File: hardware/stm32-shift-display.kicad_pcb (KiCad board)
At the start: 2 copper layers, 93.5 x 48.3 mm, 117 parts, among them J1 HDR_SWD, J2 USB_C_Receptacle_USB2.0_16P, SW1 SW_PUSH, SW2 SW_PUSH, SW3 SW_PUSH, SW4 SW_PUSH, SW5 218-2LPSTR, U1 AMS1117-3.3, U10 74HC595, U11 74HC595, U12 SM420561N, U13 SM420561N, U14 SM420561N, U2 STM32F103C8T6, U3 74HC595, U4 74HC595, U5 74HC595, U6 SM420561N, U7 SM420561N, U8 SM420561N, U9 74HC595, X1 OT32258MJBA4SL, X2 OK322532.768KJBA4SL

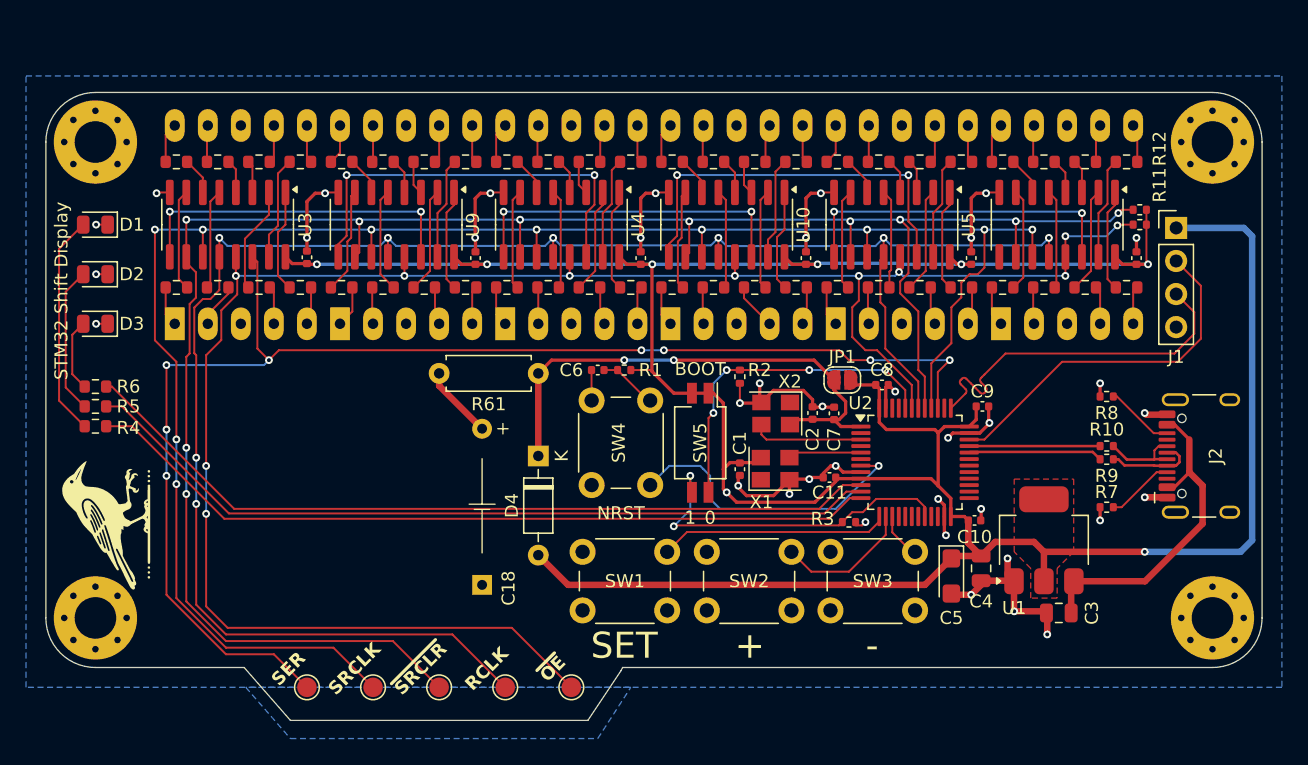
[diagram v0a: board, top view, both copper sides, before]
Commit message: Pre-autoroute on rev2
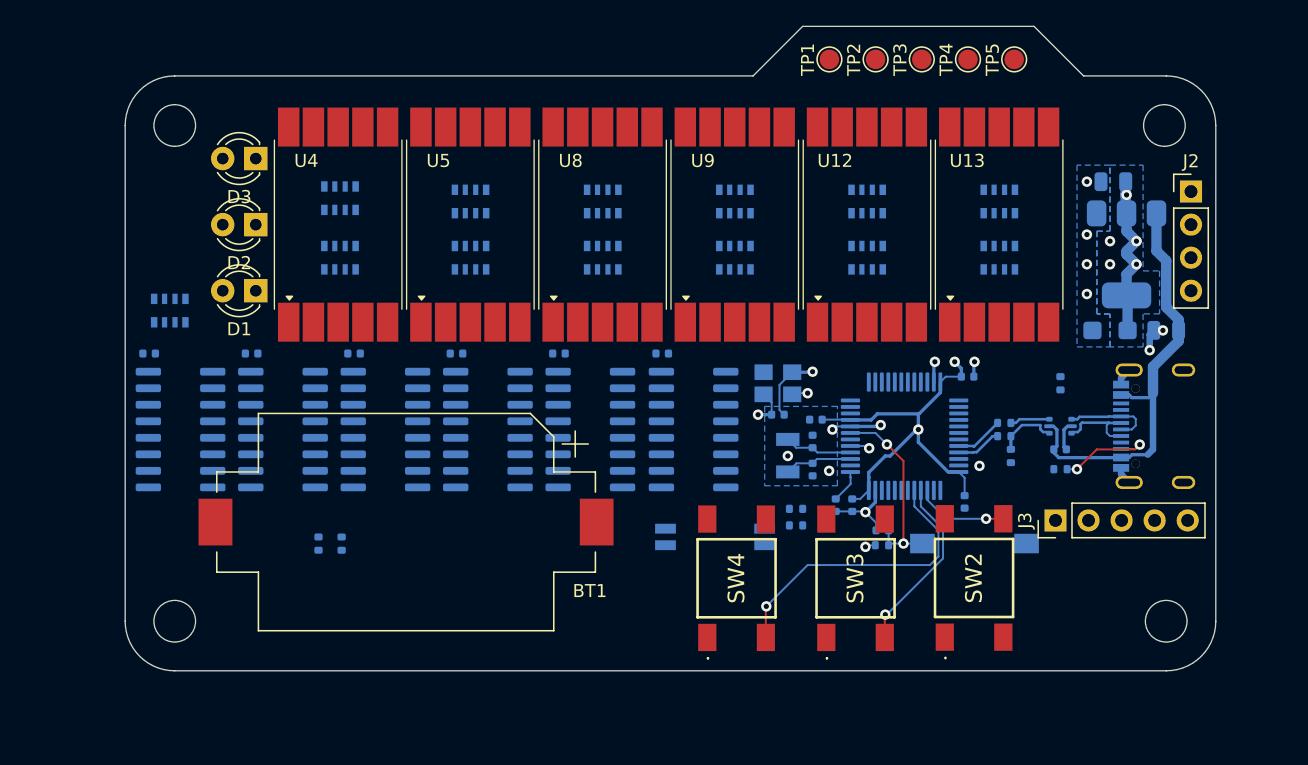
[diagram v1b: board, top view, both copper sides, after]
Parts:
- removed D4: BAT43, Diode_THT:D_DO-35_SOD27_P7.62mm_Horizontal
- removed G***: LOGO, CustomSymbols:GrackleLogo12mm
- removed JP1: SolderJumper_2_Open, Jumper:SolderJumper-2_P1.3mm_Open_RoundedPad1.0x1.5mm
- removed R10, R9: 10R, Resistor_SMD:R_0402_1005Metric
- removed R11: 10k, Resistor_SMD:R_0402_1005Metric
- removed R14, R15, R16, R17, R18, R19, R20, R21, R22, R23, R24, R25, R26, R27, R28, R29, R30, R31, R32, R33, R34, R35, R36, R37, R38, R39, R40, R41, R42, R43, R44, R45, R46, R47, R48, R49, R50, R51, R52, R53, R54, R55, R56, R57, R58, R59, R60: 470R, Resistor_SMD:R_0603_1608Metric
- removed R61: 22R, Resistor_THT:R_Axial_DIN0207_L6.3mm_D2.5mm_P7.62mm_Horizontal
- removed X2: OK322532.768KJBA4SL, Crystal:Crystal_SMD_3225-4Pin_3.2x2.5mm
- added BT1: 1060TR, Battery:BatteryHolder_Keystone_1060_1x2032, F.Cu at (144.8, 91.4)
- added C19: 100n, Capacitor_SMD:C_0402_1005Metric, B.Cu at (164.5, 78.5)
- added J3: HDR_UART, Connector_PinHeader_2.54mm:PinHeader_1x05_P2.54mm_Vertical, F.Cu at (194.7, 91.3)
- added RN1: 220R, Resistor_SMD:R_Array_Convex_4x0603, B.Cu at (139.7, 71.1)
- added RN10: 220R, Resistor_SMD:R_Array_Convex_4x0603, B.Cu at (190.4, 71.1)
- added RN11: 220R, Resistor_SMD:R_Array_Convex_4x0603, B.Cu at (180.2, 66.8)
- added RN12: 220R, Resistor_SMD:R_Array_Convex_4x0603, B.Cu at (190.4, 66.8)
- added RN13: 220R, Resistor_SMD:R_Array_Convex_4x0603, B.Cu at (126.6, 75.2)
- added RN2: 220R, Resistor_SMD:R_Array_Convex_4x0603, B.Cu at (149.7, 71.1)
- added RN3: 220R, Resistor_SMD:R_Array_Convex_4x0603, B.Cu at (139.7, 66.5)
- added RN4: 220R, Resistor_SMD:R_Array_Convex_4x0603, B.Cu at (149.7, 66.8)
- added RN5: 220R, Resistor_SMD:R_Array_Convex_4x0603, B.Cu at (159.9, 71.1)
- added RN6: 220R, Resistor_SMD:R_Array_Convex_4x0603, B.Cu at (170.1, 71.1)
- added RN7: 220R, Resistor_SMD:R_Array_Convex_4x0603, B.Cu at (159.9, 66.8)
- added RN8: 220R, Resistor_SMD:R_Array_Convex_4x0603, B.Cu at (170.1, 66.8)
- added RN9: 220R, Resistor_SMD:R_Array_Convex_4x0603, B.Cu at (180.2, 71.1)
- added U15: 74HC595, Package_SO:SOIC-16_3.9x9.9mm_P1.27mm, B.Cu at (166.9, 84.3)
- added Y1: Q13FC13500002, Crystal:Crystal_SMD_3215-2Pin_3.2x1.5mm, B.Cu at (174.1, 86.3)
- C1, C14, C15, C16, C17, C2, C6, C7, C8, R1, R12, SW5, U10, U11, U2, X1: moved to B.Cu
- C10, C9: value 100n -> 6p; moved to B.Cu
- C11, C12: footprint Capacitor_SMD:C_0402_1005Metric -> Capacitor_SMD:C_0805_2012Metric; moved to B.Cu
- C13: value 100n -> 10u; footprint Capacitor_SMD:C_0402_1005Metric -> Capacitor_Tantalum_SMD:CP_EIA-3216-18_Kemet-A; moved to B.Cu
- C18: value SCMR22C155PRBA0 -> 100n; footprint Mouser:SCMR22C155PRBA0 -> Capacitor_SMD:C_0402_1005Metric; moved to B.Cu
- C3, C4: footprint Capacitor_SMD:C_0805_2012Metric -> Capacitor_SMD:C_0402_1005Metric; moved to B.Cu
- C5: value 10u -> 100n; footprint Capacitor_Tantalum_SMD:CP_EIA-3216-18_Kemet-A -> Capacitor_SMD:C_0402_1005Metric; moved to B.Cu
- D1, D2, D3: value KT-0805Y -> LED_YLW; footprint LED_SMD:LED_0805_2012Metric -> LED_THT:LED_D3.0mm
- H1, H2, H3, H4: footprint MountingHole:MountingHole_3.2mm_M3_Pad_Via -> MountingHole:MountingHole_3.2mm_M3_ISO7380
- J1: value HDR_SWD -> GT-USB-7010ASV; footprint Connector_PinHeader_2.54mm:PinHeader_1x04_P2.54mm_Vertical -> easyeda2kicad:USB-C-SMD_G-SWITCH_GT-USB-7010ASV; moved to B.Cu
- J2: value USB_C_Receptacle_USB2.0_16P -> HDR_SWD; footprint Connector_USB:USB_C_Receptacle_HCTL_HC-TYPE-C-16P-01A -> Connector_PinHeader_2.54mm:PinHeader_1x04_P2.54mm_Vertical
- R13: value 470R -> 10k; footprint Resistor_SMD:R_0603_1608Metric -> Resistor_SMD:R_0402_1005Metric; moved to B.Cu
- R2, R3: value 10k -> 5k1; moved to B.Cu
- R4, R5: value 220R -> 0R; footprint Resistor_SMD:R_0603_1608Metric -> Resistor_SMD:R_0402_1005Metric; moved to B.Cu
- R6: value 220R -> 1k5; footprint Resistor_SMD:R_0603_1608Metric -> Resistor_SMD:R_0402_1005Metric; moved to B.Cu
- R7, R8: value 5k1 -> 10k; moved to B.Cu
- SW1: value SW_PUSH -> TS-1101-C-W; footprint Button_Switch_THT:SW_PUSH_6mm -> easyeda2kicad:SW-SMD_L6.0-W3.3-LS8.0; moved to B.Cu
- SW2, SW3, SW4: footprint Button_Switch_THT:SW_PUSH_6mm -> Mouser:TS046643BK160SMT
- U1: value AMS1117-3.3 -> USBLC6-2P6; footprint Package_TO_SOT_SMD:SOT-223-3_TabPin2 -> Package_TO_SOT_SMD:SOT-666; moved to B.Cu
- U12, U13, U8: value SM420561N -> VDMY10C0; footprint Display_7Segment:7SegmentLED_LTS6760_LTS6780 -> Mouser:VDMx10x0
- U14, U6, U7: value SM420561N -> 74HC595; footprint Display_7Segment:7SegmentLED_LTS6760_LTS6780 -> Package_SO:SOIC-16_3.9x9.9mm_P1.27mm; moved to B.Cu
- U3: value 74HC595 -> AMS1117-3.3; footprint Package_SO:SOIC-16_3.9x9.9mm_P1.27mm -> Package_TO_SOT_SMD:SOT-223-3_TabPin2; moved to B.Cu
- U4, U5, U9: value 74HC595 -> VDMY10C0; footprint Package_SO:SOIC-16_3.9x9.9mm_P1.27mm -> Mouser:VDMx10x0
- moved H4 82.3 mm to (203.2, 99.1)
- moved H3 79.8 mm to (127.0, 99.1)
- moved R6 70.6 mm to (191.3, 86.4), turned to 90 degrees
- moved R5 69.9 mm to (190.8, 84.8)
- moved R4 69.9 mm to (190.8, 83.8)
- moved U3 69.1 mm to (200.2, 70.9)
- moved R12 68.1 mm to (138.0, 93.1), turned to -90 degrees
- moved TP1 62.8 mm to (177.3, 55.9), turned to 90 degrees
- moved C12 62.2 mm to (199.1, 65.3), turned to 180 degrees
- moved TP2 61.8 mm to (180.9, 55.9), turned to 90 degrees
- moved TP3 60.9 mm to (184.4, 55.9), turned to 90 degrees
- moved TP4 59.9 mm to (188.0, 55.9), turned to 90 degrees
- moved TP5 59.1 mm to (191.5, 55.9), turned to 90 degrees
- moved C17 52.8 mm to (148.7, 78.5), turned to 180 degrees
- moved C13 49.1 mm to (198.9, 76.7), turned to 180 degrees
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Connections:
- C1 pad 1: VCC -> VBAT
- C10 pad 1: VCC -> GND
- C10 pad 2: GND -> /OSC32_OUT
- C11 pad 1: VCC -> VBUS
- C18 pad 1: Net-(C18-Pad1) -> VCC
- C2 pad 1: VBAT -> VCC
- C3 pad 1: VBUS -> VCC
- C7 pad 1: VBAT -> VCC
- C8 pad 1: VCC -> VBUS
- C9 pad 1: VCC -> GND
- C9 pad 2: GND -> /OSC32_IN
- J1 pad 1: VCC -> GND
- J1 pad 2: /SWDIO -> GND
- J1 pad 3: /SWCLK -> GND
- R12 pad 2: /Shift Display/~{SRCLR} -> /Shift Display/~{OE}
- R13 pad 1: /Shift Display/Q1A -> VCC
- R13 pad 2: /Shift Display/D1B -> /Shift Display/~{SRCLR}
- R2 pad 2: /BOOT0 -> /CC1
- R3 pad 2: /BOOT1 -> /CC2
- R4 pad 1: /LED1r -> /MCU_D-
- R4 pad 2: /LED1 -> /ESD_D-
- R5 pad 1: /LED2r -> /MCU_D+
- R5 pad 2: /LED2 -> /ESD_D+
- R6 pad 1: /LED3r -> VCC
- R6 pad 2: /LED3 -> /ESD_D+
- R7 pad 2: /CC1 -> /BOOT0
- R8 pad 2: /CC2 -> /BOOT1
- SW1 pad 2: /BTN1 -> /NRST
- SW2 pad 2: /BTN2 -> /BTN1
- SW3 pad 2: /BTN3 -> /BTN2
- SW4 pad 2: /NRST -> /BTN3
- U1 pad 1: GND -> /USB_D-
- U1 pad 2: VCC -> GND
- U1 pad 3: VBUS -> /USB_D+
- U10 pad 1: /Shift Display/Q4B -> /Shift Display/Q3B
- U10 pad 14: /Shift Display/SER3 -> /Shift Display/SER2
- U10 pad 15: /Shift Display/Q4A -> /Shift Display/Q3A
- U10 pad 2: /Shift Display/Q4C -> /Shift Display/Q3C
- U10 pad 3: /Shift Display/Q4D -> /Shift Display/Q3D
- U10 pad 4: /Shift Display/Q4E -> /Shift Display/Q3E
- U10 pad 5: /Shift Display/Q4F -> /Shift Display/Q3F
- U10 pad 6: /Shift Display/Q4G -> /Shift Display/Q3G
- U10 pad 7: /Shift Display/Q4H -> /Shift Display/Q3H
- U10 pad 9: /Shift Display/SER4 -> /Shift Display/SER3
- U11 pad 1: /Shift Display/Q6B -> /Shift Display/Q4B
- U11 pad 14: /Shift Display/SER5 -> /Shift Display/SER3
- U11 pad 15: /Shift Display/Q6A -> /Shift Display/Q4A
- U11 pad 2: /Shift Display/Q6C -> /Shift Display/Q4C
- U11 pad 3: /Shift Display/Q6D -> /Shift Display/Q4D
- U11 pad 4: /Shift Display/Q6E -> /Shift Display/Q4E
- U11 pad 5: /Shift Display/Q6F -> /Shift Display/Q4F
- U11 pad 6: /Shift Display/Q6G -> /Shift Display/Q4G
- U11 pad 7: /Shift Display/Q6H -> /Shift Display/Q4H
- U11 pad 9: unconnected-(U11-QH'-Pad9) -> /Shift Display/SER4
- U12 pad 1: /Shift Display/D2E -> /Shift Display/D5E
- U12 pad 10: /Shift Display/D2G -> /Shift Display/D5G
- U12 pad 2: /Shift Display/D2D -> /Shift Display/D5D
- U12 pad 4: /Shift Display/D2C -> /Shift Display/D5C
- U12 pad 5: /Shift Display/D2P -> /Shift Display/D5P
- U12 pad 6: /Shift Display/D2B -> /Shift Display/D5B
- U12 pad 7: /Shift Display/D2A -> /Shift Display/D5A
- U12 pad 9: /Shift Display/D2F -> /Shift Display/D5F
- U13 pad 1: /Shift Display/D4E -> /Shift Display/D6E
- U13 pad 10: /Shift Display/D4G -> /Shift Display/D6G
- U13 pad 2: /Shift Display/D4D -> /Shift Display/D6D
- U13 pad 4: /Shift Display/D4C -> /Shift Display/D6C
- U13 pad 5: /Shift Display/D4P -> /Shift Display/D6P
- U13 pad 6: /Shift Display/D4B -> /Shift Display/D6B
- U13 pad 7: /Shift Display/D4A -> /Shift Display/D6A
- U13 pad 9: /Shift Display/D4F -> /Shift Display/D6F
- U14 pad 1: /Shift Display/D6E -> /Shift Display/Q5B
- U14 pad 10: /Shift Display/D6G -> /Shift Display/~{SRCLR}
- U14 pad 2: /Shift Display/D6D -> /Shift Display/Q5C
- U14 pad 3: GND -> /Shift Display/Q5D
- U14 pad 4: /Shift Display/D6C -> /Shift Display/Q5E
- U14 pad 5: /Shift Display/D6P -> /Shift Display/Q5F
- U14 pad 6: /Shift Display/D6B -> /Shift Display/Q5G
- U14 pad 7: /Shift Display/D6A -> /Shift Display/Q5H
- U14 pad 9: /Shift Display/D6F -> /Shift Display/SER5
- U2 pad 10: /LED3 -> /Shift Display/~{OE}
- U2 pad 11: /LED2 -> /Shift Display/~{SRCLR}
- U2 pad 12: /LED1 -> /Shift Display/RCLK
- U2 pad 13: /BTN1 -> /Shift Display/SER
- U2 pad 14: /BTN2 -> /Shift Display/SRCLK
- U2 pad 15: /BTN3 -> unconnected-(U2-PA5-Pad15)
- U2 pad 21: unconnected-(U2-PB10-Pad21) -> /TX3
- U2 pad 22: unconnected-(U2-PB11-Pad22) -> /RX3
- U2 pad 26: unconnected-(U2-PB13-Pad26) -> /CTS3
- U2 pad 27: unconnected-(U2-PB14-Pad27) -> /RTS3
- U2 pad 39: /Shift Display/SER -> /BTN1
- U2 pad 4: unconnected-(U2-PC15-Pad4) -> /OSC32_OUT
- U2 pad 40: /Shift Display/SRCLK -> /BTN2
- U2 pad 41: /Shift Display/~{SRCLR} -> /BTN3
- U2 pad 42: /Shift Display/RCLK -> /LED1
- U2 pad 43: /Shift Display/~{OE} -> /LED2
- U2 pad 45: unconnected-(U2-PB8-Pad45) -> /LED3
- U3 pad 1: /Shift Display/Q1B -> GND
- U3 pad 2: /Shift Display/Q1C -> VCC
- U3 pad 3: /Shift Display/Q1D -> VBUS
- U4 pad 1: /Shift Display/Q3B -> /Shift Display/D1E
- U4 pad 10: /Shift Display/~{SRCLR} -> /Shift Display/D1G
- U4 pad 2: /Shift Display/Q3C -> /Shift Display/D1D
- U4 pad 3: /Shift Display/Q3D -> GND
- U4 pad 4: /Shift Display/Q3E -> /Shift Display/D1C
- U4 pad 5: /Shift Display/Q3F -> /Shift Display/D1P
- U4 pad 6: /Shift Display/Q3G -> /Shift Display/D1B
- U4 pad 7: /Shift Display/Q3H -> /Shift Display/D1A
- U4 pad 9: /Shift Display/SER3 -> /Shift Display/D1F
- U5 pad 1: /Shift Display/Q5B -> /Shift Display/D2E
- U5 pad 10: /Shift Display/~{SRCLR} -> /Shift Display/D2G
- U5 pad 2: /Shift Display/Q5C -> /Shift Display/D2D
- U5 pad 3: /Shift Display/Q5D -> GND
- U5 pad 4: /Shift Display/Q5E -> /Shift Display/D2C
- U5 pad 5: /Shift Display/Q5F -> /Shift Display/D2P
- U5 pad 6: /Shift Display/Q5G -> /Shift Display/D2B
- U5 pad 7: /Shift Display/Q5H -> /Shift Display/D2A
- U5 pad 9: /Shift Display/SER5 -> /Shift Display/D2F
- U6 pad 1: /Shift Display/D1E -> /Shift Display/Q1B
- U6 pad 10: /Shift Display/D1G -> /Shift Display/~{SRCLR}
- U6 pad 2: /Shift Display/D1D -> /Shift Display/Q1C
- U6 pad 3: GND -> /Shift Display/Q1D
- U6 pad 4: /Shift Display/D1C -> /Shift Display/Q1E
- U6 pad 5: /Shift Display/D1P -> /Shift Display/Q1F
- U6 pad 6: /Shift Display/D1B -> /Shift Display/Q1G
- U6 pad 7: /Shift Display/D1A -> /Shift Display/Q1H
- U6 pad 9: /Shift Display/D1F -> /Shift Display/SER1
- U7 pad 1: /Shift Display/D3E -> /Shift Display/Q2B
- U7 pad 10: /Shift Display/D3G -> /Shift Display/~{SRCLR}
- U7 pad 2: /Shift Display/D3D -> /Shift Display/Q2C
- U7 pad 3: GND -> /Shift Display/Q2D
- U7 pad 4: /Shift Display/D3C -> /Shift Display/Q2E
- U7 pad 5: /Shift Display/D3P -> /Shift Display/Q2F
- U7 pad 6: /Shift Display/D3B -> /Shift Display/Q2G
- U7 pad 7: /Shift Display/D3A -> /Shift Display/Q2H
- U7 pad 9: /Shift Display/D3F -> /Shift Display/SER2
- U8 pad 1: /Shift Display/D5E -> /Shift Display/D3E
- U8 pad 10: /Shift Display/D5G -> /Shift Display/D3G
- U8 pad 2: /Shift Display/D5D -> /Shift Display/D3D
- U8 pad 4: /Shift Display/D5C -> /Shift Display/D3C
- U8 pad 5: /Shift Display/D5P -> /Shift Display/D3P
- U8 pad 6: /Shift Display/D5B -> /Shift Display/D3B
- U8 pad 7: /Shift Display/D5A -> /Shift Display/D3A
- U8 pad 9: /Shift Display/D5F -> /Shift Display/D3F
- U9 pad 1: /Shift Display/Q2B -> /Shift Display/D4E
- U9 pad 10: /Shift Display/~{SRCLR} -> /Shift Display/D4G
- U9 pad 2: /Shift Display/Q2C -> /Shift Display/D4D
- U9 pad 3: /Shift Display/Q2D -> GND
- U9 pad 4: /Shift Display/Q2E -> /Shift Display/D4C
- U9 pad 5: /Shift Display/Q2F -> /Shift Display/D4P
- U9 pad 6: /Shift Display/Q2G -> /Shift Display/D4B
- U9 pad 7: /Shift Display/Q2H -> /Shift Display/D4A
- U9 pad 9: /Shift Display/SER2 -> /Shift Display/D4F
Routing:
- net VCC: track 244.8 -> 46.8 mm, vias 8 -> 9
- net /Shift Display/~{SRCLR}: track 155.0 -> 0.00 mm, vias 10 -> 0
- net /Shift Display/~{OE}: track 149.5 -> 0.00 mm, vias 11 -> 0
- net /Shift Display/SRCLK: track 142.7 -> 0.00 mm, vias 10 -> 0
- net /Shift Display/RCLK: track 142.3 -> 0.00 mm, vias 8 -> 0
- net /Shift Display/SER: track 104.9 -> 0.00 mm, vias 8 -> 0
- net GND: track 94.6 -> 25.5 mm, vias 37 -> 15
- net /LED3: track 62.7 -> 0.00 mm
- net /LED2: track 62.1 -> 0.00 mm
- net /LED1: track 61.6 -> 0.00 mm
- net VBAT: track 39.4 -> 2.55 mm, vias 2 -> 0
- net /Shift Display/SER2: track 32.1 -> 0.00 mm, vias 2 -> 0
- net /Shift Display/SER4: track 30.9 -> 0.00 mm, vias 2 -> 0
- net /SWCLK: track 28.0 -> 0.00 mm
- net /SWDIO: track 27.8 -> 0.00 mm
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- added copper zone on In1.Cu, net GND
- added copper zone on B.Cu, net VCC
- added copper zone on In2.Cu, net VCC
- removed copper zone on F.Cu, net VCC
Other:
- board size 93.5 x 48.3 mm -> 83.8 x 49.5 mm
- copper layers 2 -> 4
- board text removed: "+"
- board text removed: "-"
- board text removed: "0"
- board text removed: "1"
- board text removed: "3V3"
- board text removed: "A"
- board text removed: "B"
- board text removed: "BOOT"
- board text removed: "C"
- board text removed: "CC"
- board text removed: "CLK"
- board text removed: "D"
- board text removed: "DIO"
- board text removed: "DP"
- board text removed: "E"
- board text removed: "F"
- board text removed: "G"
- board text removed: "GND"
- board text removed: "JLCJLCJLC"
- board text removed: "NRST"
- board text removed: "RCLK"
- board text removed: "SER"
- board text removed: "SET"
- board text removed: "SRCLK"
- board text removed: "STM32 Shift Display"
- board text removed: "rev 0"
- board text removed: "~{OE}"
- board text removed: "~{SRCLR}"
